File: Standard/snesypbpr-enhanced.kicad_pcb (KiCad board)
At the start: 2 copper layers, 31.9 x 21.6 mm, 15 parts, among them J1 Pr In, J2 Pb In, J3 +5V, J4 GND, J5 Pr Out, J6 Pb Out, Q1 S8050/SS8050

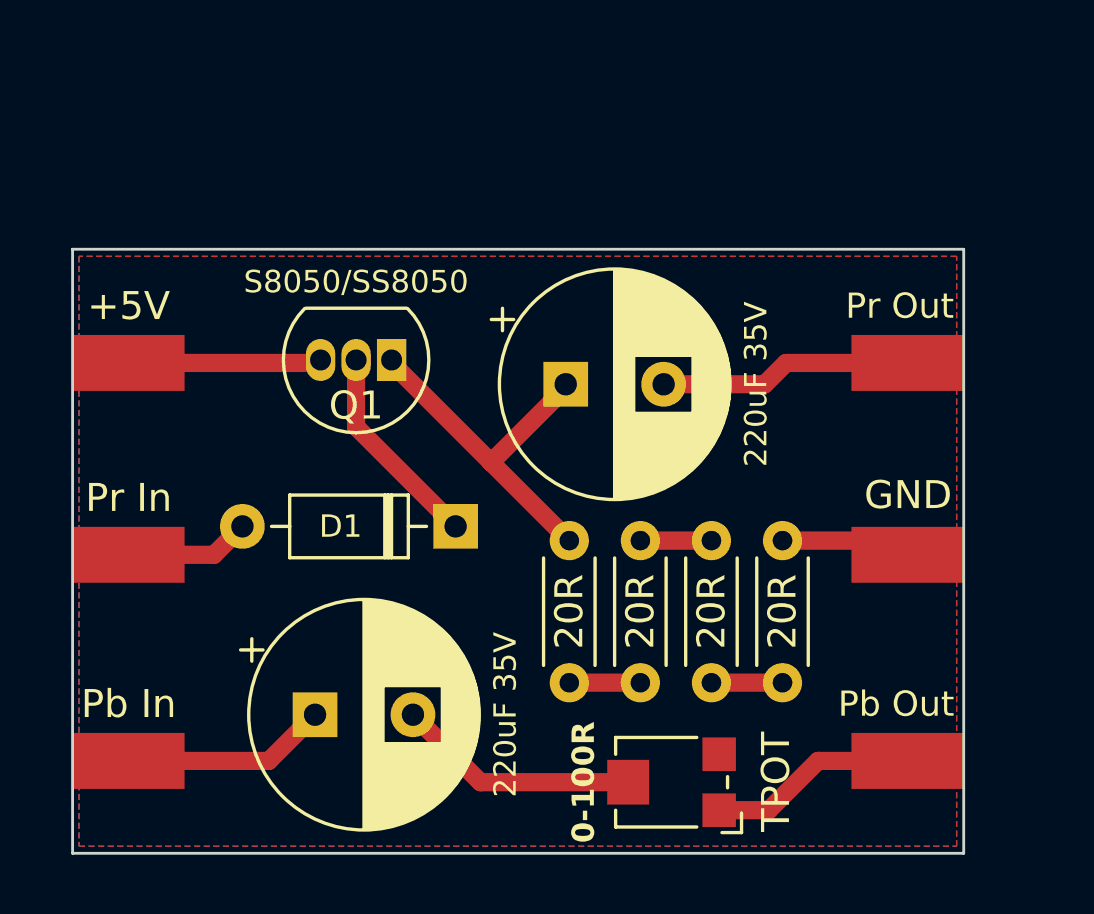
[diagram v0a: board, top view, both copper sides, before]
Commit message: 2.0
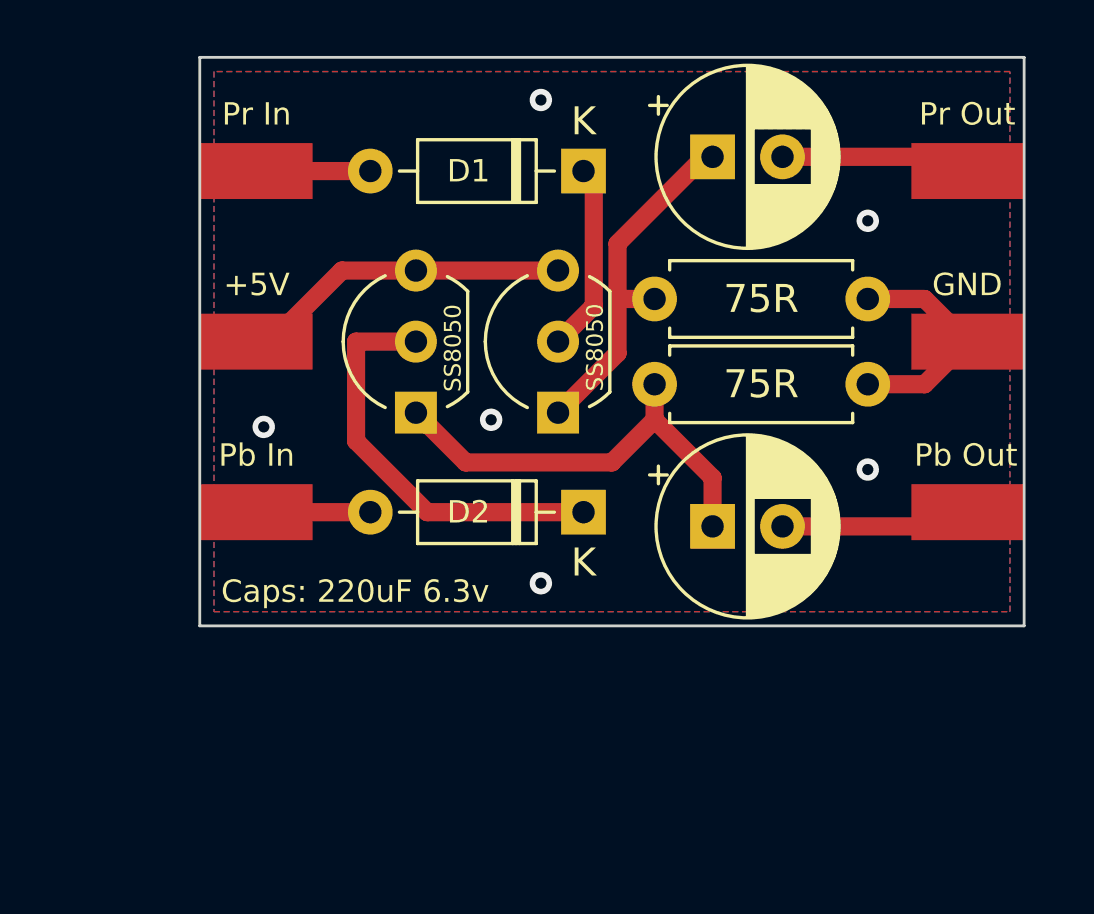
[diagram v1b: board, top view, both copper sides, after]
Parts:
- removed R3, R4: 20R, Resistor_THT:R_Axial_DIN0204_L3.6mm_D1.6mm_P5.08mm_Horizontal
- removed RV1: 0-100R, Potentiometer_SMD:Potentiometer_Bourns_TC33X_Vertical
- added D2: 1N4148, Diode_THT:D_DO-35_SOD27_P7.62mm_Horizontal, F.Cu at (123.4, 70.6)
- added Q2: S8050/SS8050, Package_TO_SOT_THT:TO-92_Inline_Wide, F.Cu at (117.5, 67.1)
- C1, C2: value 220uF 35V -> 220uF 6.3V; footprint Capacitor_THT:CP_Radial_D8.0mm_P3.50mm -> Capacitor_THT:CP_Radial_D6.3mm_P2.50mm
- Q1: footprint Package_TO_SOT_THT:TO-92_Inline -> Package_TO_SOT_THT:TO-92_Inline_Wide
- R1, R2: value 20R -> 75R; footprint Resistor_THT:R_Axial_DIN0204_L3.6mm_D1.6mm_P5.08mm_Horizontal -> Resistor_THT:R_Axial_DIN0207_L6.3mm_D2.5mm_P7.62mm_Horizontal
- moved C2 15.7 mm to (128.1, 71.1)
- moved J1 14.5 mm to (111.8, 58.4), turned to 90 degrees
- moved D1 13.5 mm to (123.4, 58.4)
- moved J2 10.00 mm to (111.8, 70.6), turned to 90 degrees
- moved C1 9.68 mm to (128.1, 57.9)
- moved R1 9.16 mm to (126.0, 63.0), turned to 0 degrees
- moved J6 9.14 mm to (137.2, 70.6)
- moved J4 7.91 mm to (137.2, 64.5)
- moved J5 7.18 mm to (137.2, 58.4)
- moved Q1 6.24 mm to (122.5, 67.1), turned to 90 degrees
- moved R2 5.61 mm to (126.0, 66.0), turned to 0 degrees
- moved J3 4.64 mm to (111.8, 64.5), turned to 90 degrees
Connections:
- C2 pad 1: Net-(J2-Pin_1) -> Net-(Q2-E)
- C2 pad 2: Net-(C2-Pad2) -> Net-(J6-Pin_1)
- J2 pad 1: Net-(J2-Pin_1) -> Net-(D2-A)
- R1 pad 2: Net-(R1-Pad2) -> GND
- R2 pad 1: Net-(R2-Pad1) -> Net-(Q2-E)
- R2 pad 2: Net-(R1-Pad2) -> GND
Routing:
- net Net-(Q2-E): track 0.00 -> 15.8 mm
- net Net-(D2-K): track 0.00 -> 14.9 mm
- net Net-(C2-Pad2): track 8.69 -> 0.00 mm
- net Net-(J2-Pin_1): track 7.35 -> 0.00 mm
- net +5V: track 6.90 -> 11.8 mm
- net Net-(D2-A): track 0.00 -> 4.06 mm
- net GND: track 4.68 -> 8.37 mm, vias 0 -> 6
- net Net-(R3-Pad2): track 2.54 -> 0.00 mm
- net Net-(R2-Pad1): track 2.54 -> 0.00 mm
- net Net-(R1-Pad2): track 2.54 -> 0.00 mm
- net Net-(J5-Pin_1): track 9.03 -> 6.81 mm
- net Net-(J6-Pin_1): track 7.46 -> 6.81 mm
- net Net-(D1-K): track 7.42 -> 6.78 mm
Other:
- board size 31.9 x 21.6 mm -> 29.5 x 20.3 mm
- board text added: "Caps: 220uF 6.3v"
- board text added: "SS8050"
- board text removed: "Original Circuit Design: NightWolve (Nicholas Livaditis) Other Credits: thesteve, Duo_R, Michael Moffitt"
- board text removed: "SNES {dblquote}Enhanced{dblquote} Component Video PCB by joshman196"
